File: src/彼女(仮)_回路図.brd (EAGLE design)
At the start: 65.7 x 51 mm, 55 parts, among them IC1 A3921, SW1 TVAF06-A020B-R, SW2 TVAF06-A020B-R, SW3 THAF01-NC-R, SW4 SS-12D00G3

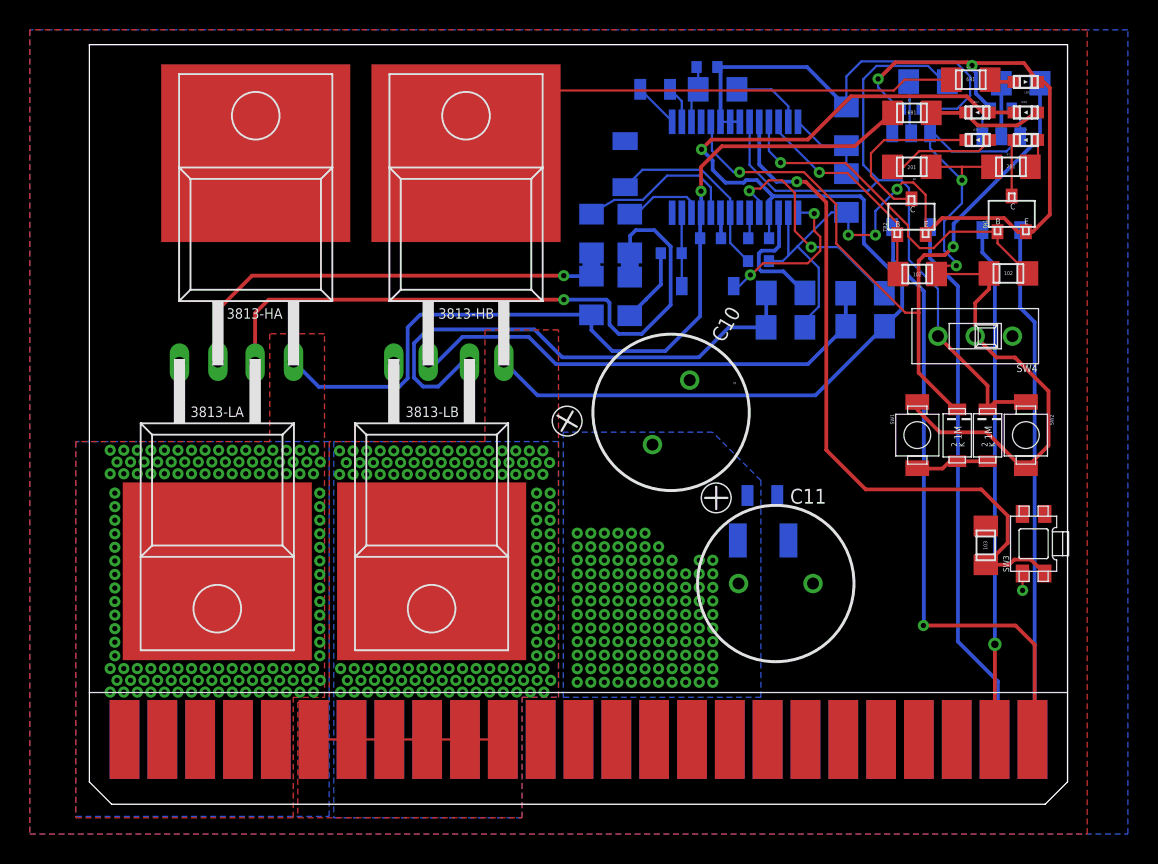
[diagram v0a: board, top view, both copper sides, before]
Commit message: 配線完了
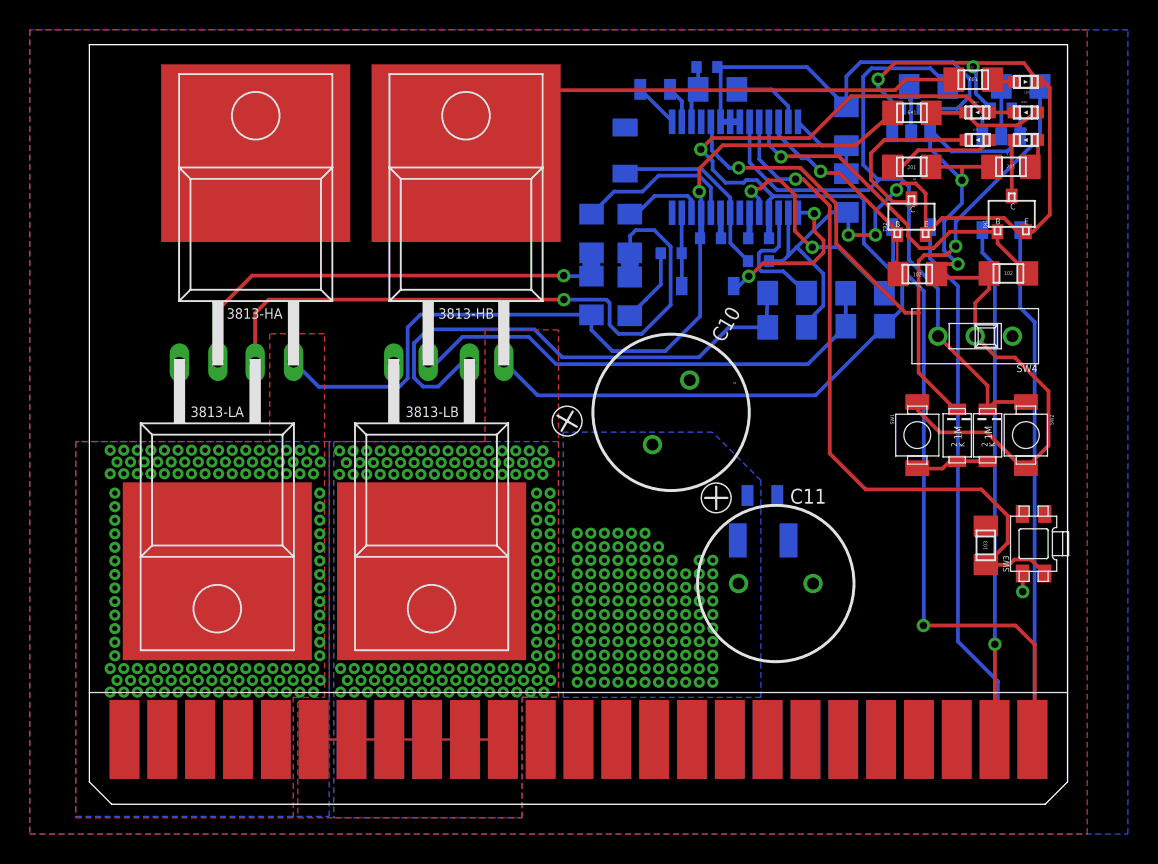
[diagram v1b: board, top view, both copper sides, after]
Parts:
- moved C9 0.91 mm to (36.0, 43.9)
- moved R9 0.32 mm to (57.6, 48.2)
- moved R1 0.21 mm to (63.8, 48.2)
- moved R22 0.16 mm to (58.0, 48.6)
- moved R18 0.11 mm to (48.1, 32.0)
- moved R10 0.10 mm to (48.1, 34.3)
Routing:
- net VCC: track 53.4 -> 53.9 mm
